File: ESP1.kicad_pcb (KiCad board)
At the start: 2 copper layers, 29.1 x 39 mm, 17 parts, among them J1 Conn_01x04_Male, J2 USB_C_Receptacle_USB2.0, U1 LM1117-3.3, U2 ESP32-S2-MINI-1-N4_EXP

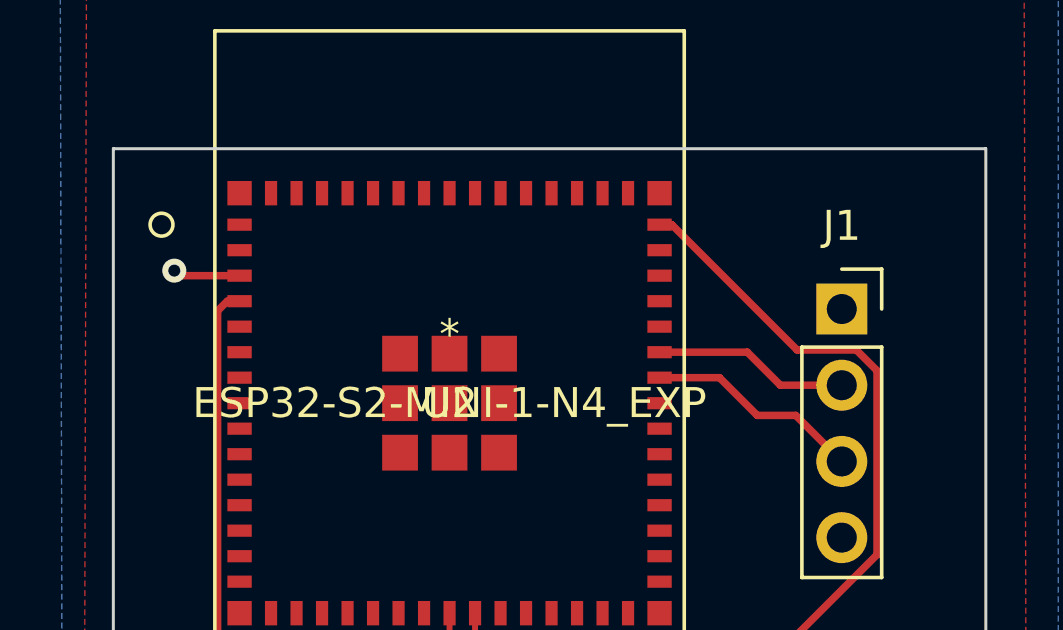
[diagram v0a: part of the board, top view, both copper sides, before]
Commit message: Works for now
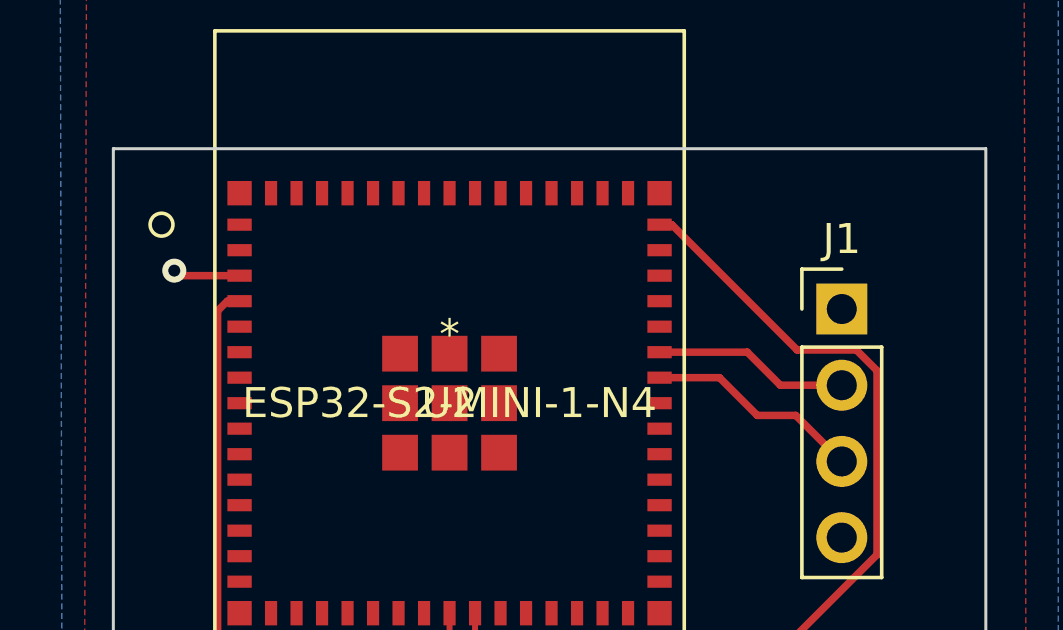
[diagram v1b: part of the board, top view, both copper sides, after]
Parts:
- J1: footprint Connector_PinSocket_2.54mm:PinSocket_1x04_P2.54mm_Vertical -> Connector_PinHeader_2.54mm:PinHeader_1x04_P2.54mm_Vertical
- U2: value ESP32-S2-MINI-1-N4_EXP -> ESP32-S2-MINI-1-N4
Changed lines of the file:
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@@
     )
   )
-  (footprint "Connector_PinSocket_2.54mm:PinSocket_1x04_P2.54mm_Vertical" (layer "F.Cu")
+  (footprint "Connector_PinHeader_2.54mm:PinHeader_1x04_P2.54mm_Vertical" (layer "F.Cu")
     (at 156.616 100.975)
-    (descr "Through hole straight socket strip, 1x04, 2.54mm pitch, single row (from Kicad 4.0.7), script generated")
-    (tags "Through hole socket strip THT 1x04 2.54mm single row")
+    (descr "Through hole straight pin header, 1x04, 2.54mm pitch, single row")
+    (tags "Through hole pin header THT 1x04 2.54mm single row")
     (property "Sheetfile" "ESP1.kicad_sch")
     (property "Sheetname" "")
     (attr through_hole)
-    (fp_text reference "J1" (at 0 -2.77) (layer "F.SilkS")
-      (effects (font (size 1 1) (thickness 0.15)))
-    )
-    (fp_text value "Conn_01x04_Male" (at 0 10.39) (layer "F.Fab")
+    (fp_text reference "J1" (at 0 -2.33) (layer "F.SilkS")
+      (effects (font (size 1 1) (thickness 0.15)))
+    )
+    (fp_text value "Conn_01x04_Male" (at 0 9.95) (layer "F.Fab")
       (effects (font (size 1 1) (thickness 0.15)))
     )
@@
       (effects (font (size 1 1) (thickness 0.15)))
     )
+    (fp_line (start -1.33 1.27) (end 1.33 1.27) (layer "F.SilkS") (width 0.12))
     (fp_line (start -1.33 8.95) (end 1.33 8.95) (layer "F.SilkS") (width 0.12))
     (fp_line (start -1.33 1.27) (end -1.33 8.95) (layer "F.SilkS") (width 0.12))
-    (fp_line (start -1.33 1.27) (end 1.33 1.27) (layer "F.SilkS") (width 0.12))
-    (fp_line (start 1.33 -1.33) (end 1.33 0) (layer "F.SilkS") (width 0.12))
+    (fp_line (start -1.33 -1.33) (end 0 -1.33) (layer "F.SilkS") (width 0.12))
     (fp_line (start 1.33 1.27) (end 1.33 8.95) (layer "F.SilkS") (width 0.12))
-    (fp_line (start 0 -1.33) (end 1.33 -1.33) (layer "F.SilkS") (width 0.12))
-    (fp_line (start 1.75 9.4) (end -1.8 9.4) (layer "F.CrtYd") (width 0.05))
-    (fp_line (start -1.8 9.4) (end -1.8 -1.8) (layer "F.CrtYd") (width 0.05))
-    (fp_line (start 1.75 -1.8) (end 1.75 9.4) (layer "F.CrtYd") (width 0.05))
-    (fp_line (start -1.8 -1.8) (end 1.75 -1.8) (layer "F.CrtYd") (width 0.05))
-    (fp_line (start -1.27 -1.27) (end 0.635 -1.27) (layer "F.Fab") (width 0.1))
-    (fp_line (start -1.27 8.89) (end -1.27 -1.27) (layer "F.Fab") (width 0.1))
+    (fp_line (start -1.33 0) (end -1.33 -1.33) (layer "F.SilkS") (width 0.12))
+    (fp_line (start 1.8 9.4) (end 1.8 -1.8) (layer "F.CrtYd") (width 0.05))
+    (fp_line (start -1.8 9.4) (end 1.8 9.4) (layer "F.CrtYd") (width 0.05))
+    (fp_line (start -1.8 -1.8) (end -1.8 9.4) (layer "F.CrtYd") (width 0.05))
+    (fp_line (start 1.8 -1.8) (end -1.8 -1.8) (layer "F.CrtYd") (width 0.05))
+    (fp_line (start 1.27 -1.27) (end 1.27 8.89) (layer "F.Fab") (width 0.1))
+    (fp_line (start -0.635 -1.27) (end 1.27 -1.27) (layer "F.Fab") (width 0.1))
+    (fp_line (start -1.27 -0.635) (end -0.635 -1.27) (layer "F.Fab") (width 0.1))
     (fp_line (start 1.27 8.89) (end -1.27 8.89) (layer "F.Fab") (width 0.1))
-    (fp_line (start 1.27 -0.635) (end 1.27 8.89) (layer "F.Fab") (width 0.1))
-    (fp_line (start 0.635 -1.27) (end 1.27 -0.635) (layer "F.Fab") (width 0.1))
+    (fp_line (start -1.27 8.89) (end -1.27 -0.635) (layer "F.Fab") (width 0.1))
     (pad "1" thru_hole rect (at 0 0) (size 1.7 1.7) (drill 1) (layers *.Cu *.Mask)
       (net 3 "+3V3") (pinfunction "Pin_1") (pintype "passive"))
@@
     (pad "4" thru_hole oval (at 0 7.62) (size 1.7 1.7) (drill 1) (layers *.Cu *.Mask)
       (net 2 "GND") (pinfunction "Pin_4") (pintype "passive"))
-    (model "${KICAD6_3DMODEL_DIR}/Connector_PinSocket_2.54mm.3dshapes/PinSocket_1x04_P2.54mm_Vertical.wrl"
+    (model "${KICAD6_3DMODEL_DIR}/Connector_PinHeader_2.54mm.3dshapes/PinHeader_1x04_P2.54mm_Vertical.wrl"
       (offset (xyz 0 0 0))
       (scale (xyz 1 1 1))
@@
       (effects (font (size 1 1) (thickness 0.15)))
     )
-    (fp_text value "ESP32-S2-MINI-1-N4_EXP" (at 0 2.288515) (layer "F.SilkS")
-      (effects (font (size 1 1) (thickness 0.15)))
-    )
+    (fp_text value "ESP32-S2-MINI-1-N4" (at 0 2.288515) (layer "F.SilkS")
+      (effects (font (size 1 1) (thickness 0.15)))
+    )
